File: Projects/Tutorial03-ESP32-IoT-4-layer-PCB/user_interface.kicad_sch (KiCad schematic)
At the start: 6 parts, among them J4 Conn_01x04_Pin, J5 Conn_01x05_Pin, Q2 BC817, Q3 BC817

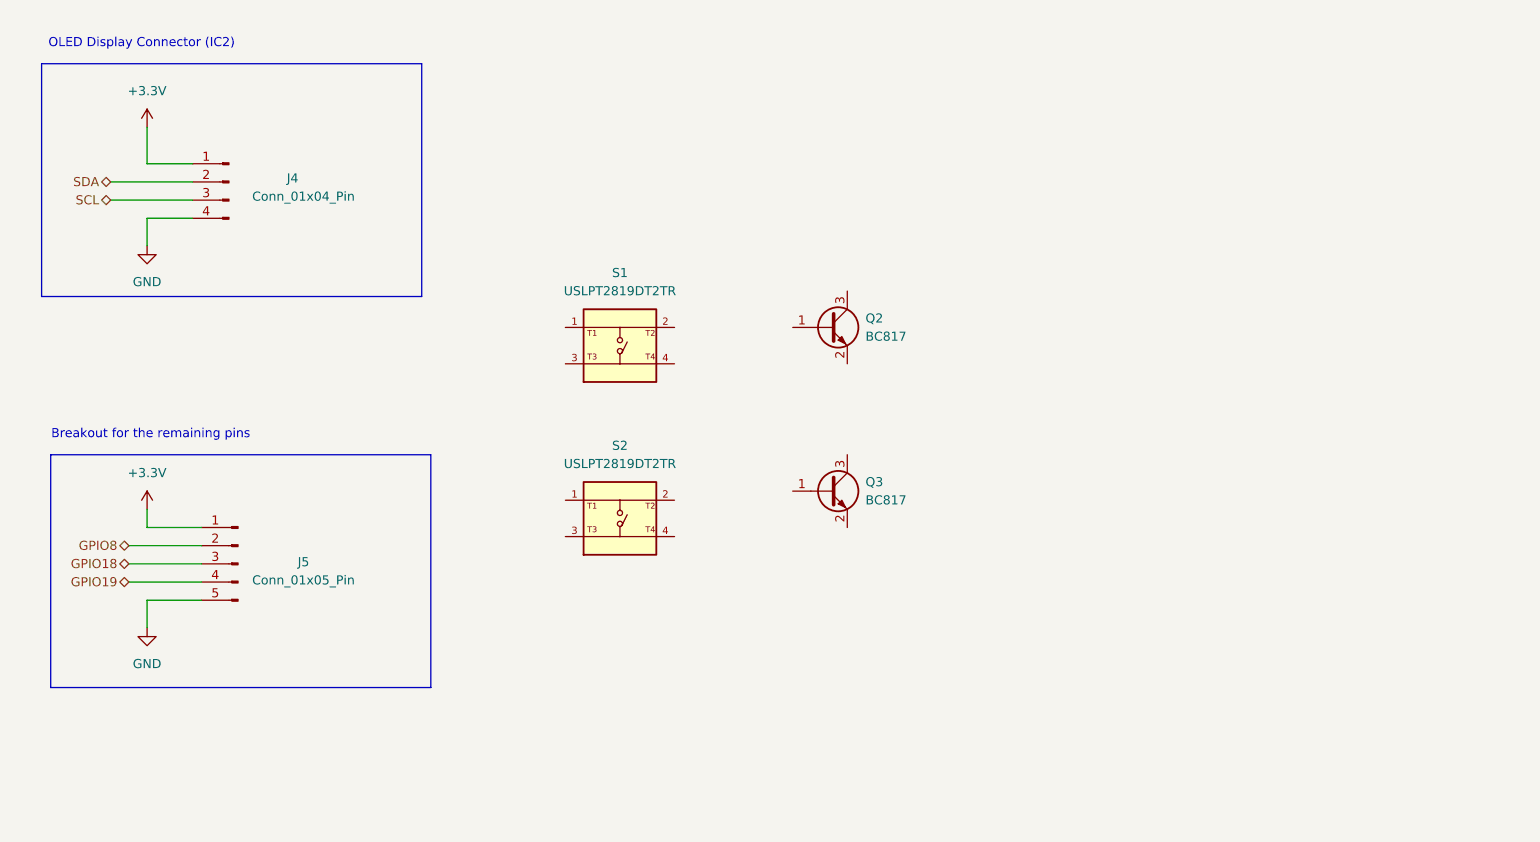
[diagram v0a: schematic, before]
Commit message: 20260329
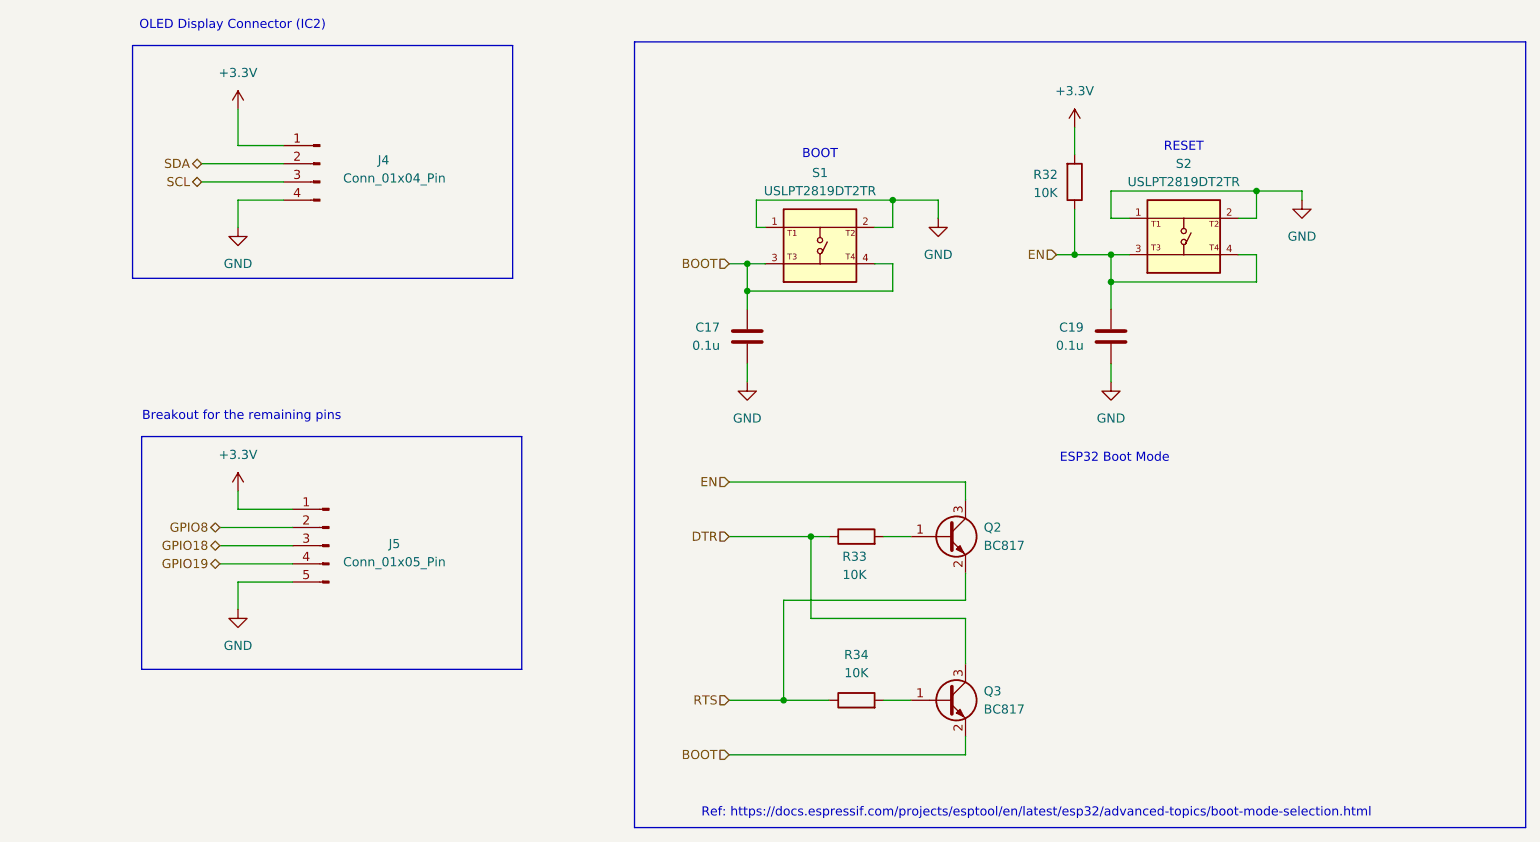
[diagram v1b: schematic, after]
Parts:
- added C17, C19: 0.1u, symbol Device:C
- added R32, R33, R34: 10K, symbol Device:R
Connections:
- net +3.3V: now also R32.2
- net GND: now also S1.1, S1.2, S2.1, S2.2, C17.2, C19.2
- net BOOT: now reaches S1.3
- net BOOT: now also Q3.2 (E), S1.4, C17.1
- net EN: now reaches S2.3
- net EN: now also Q2.3 (C), S2.4, C19.1, R32.1
- net at Q2.1 (B): now also R33.2
- net RTS: now reaches Q2.2 (E)
- net RTS: now also R34.1
- net at Q3.1 (B): now also R34.2
- net DTR: now reaches Q3.3 (C)
- net DTR: now also R33.1
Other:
- note added: "BOOT"
- note added: "ESP32 Boot Mode"
- note added: "RESET"
- note added: "Ref: https://docs.espressif.com/projects/esptool/en/latest/esp32/advanced-topics/boot-mode-selection.html"
- moved on the sheet: J4, J5, Q2, Q3, S1, S2

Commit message: 20260425
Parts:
- C17, C19: footprint (none) -> Capacitor_SMD:C_0805_2012Metric
- J4: footprint (none) -> Connector_PinHeader_2.54mm:PinHeader_1x04_P2.54mm_Vertical
- J5: footprint (none) -> Connector_PinHeader_2.54mm:PinHeader_1x05_P2.54mm_Vertical
- R32, R33, R34: footprint (none) -> Resistor_SMD:R_0805_2012Metric
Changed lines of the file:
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@@
 			)
 		)
-		(property "Footprint" ""
+		(property "Footprint" "Capacitor_SMD:C_0805_2012Metric"
 			(at 138.1252 91.44 0)
 			(effects
@@
 			)
 		)
-		(property "Footprint" ""
+		(property "Footprint" "Connector_PinHeader_2.54mm:PinHeader_1x04_P2.54mm_Vertical"
 			(at 77.47 63.5 0)
 			(effects
@@
 			)
 		)
-		(property "Footprint" ""
+		(property "Footprint" "Resistor_SMD:R_0805_2012Metric"
 			(at 181.102 66.04 90)
 			(effects
@@
 			)
 		)
-		(property "Footprint" ""
+		(property "Footprint" "Capacitor_SMD:C_0805_2012Metric"
 			(at 188.9252 91.44 0)
 			(effects
@@
 			)
 		)
-		(property "Footprint" ""
+		(property "Footprint" "Connector_PinHeader_2.54mm:PinHeader_1x05_P2.54mm_Vertical"
 			(at 78.74 116.84 0)
 			(effects
@@
 			)
 		)
-		(property "Footprint" ""
+		(property "Footprint" "Resistor_SMD:R_0805_2012Metric"
 			(at 152.4 117.348 90)
 			(effects
@@
 			)
 		)
-		(property "Footprint" ""
+		(property "Footprint" "Resistor_SMD:R_0805_2012Metric"
 			(at 152.4 140.208 90)
 			(effects
